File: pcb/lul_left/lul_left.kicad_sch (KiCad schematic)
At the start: 42 parts, among them J1 JST Connector, J2 JST Connector, SW1 SW_Push, SW10 SW_Push, SW11 SW_Push, SW12 SW_Push, SW13 SW_Push, SW14 SW_Push, SW15 SW_Push, SW16 SW_Push, SW17 SW_Push, SW18 SW_Push, SW19 SW_Push, SW2 SW_Push, SW20 SW_Push, SW21 SW_Push, SW22 SW_Push, SW23 SW_Push, SW24 SW_Push, SW25 SW_Push, SW26 SW_Push, SW27 SW_Push, SW28 SW_Push, SW29 SW_Push, SW3 SW_Push, SW30 SW_Push, SW31 SW_Push, SW32 SW_Push, SW33 SW_Push, SW34 SW_Push, SW4 SW_Push, SW5 SW_Push, SW6 SW_Push, SW7 SW_Push, SW8 SW_Push, SW9 SW_Push, U1 nice_nano, U2 nice_nano

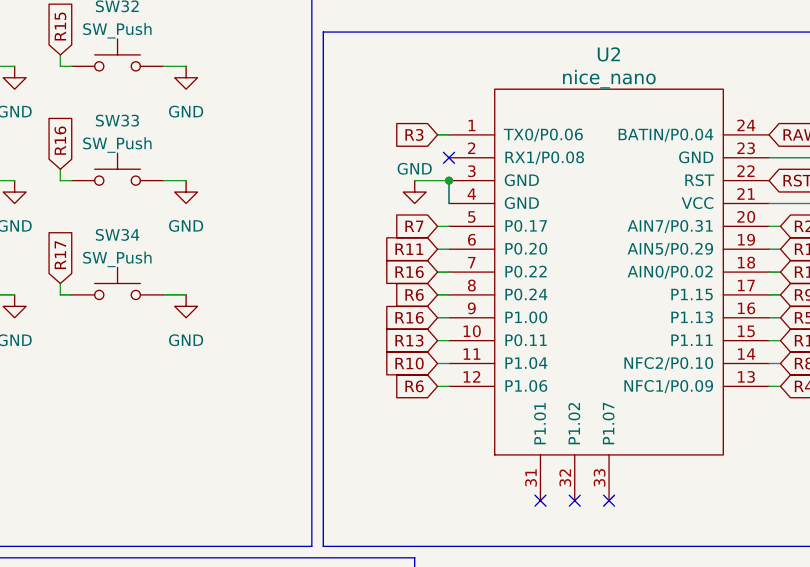
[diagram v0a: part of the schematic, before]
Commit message: fix small connection issue
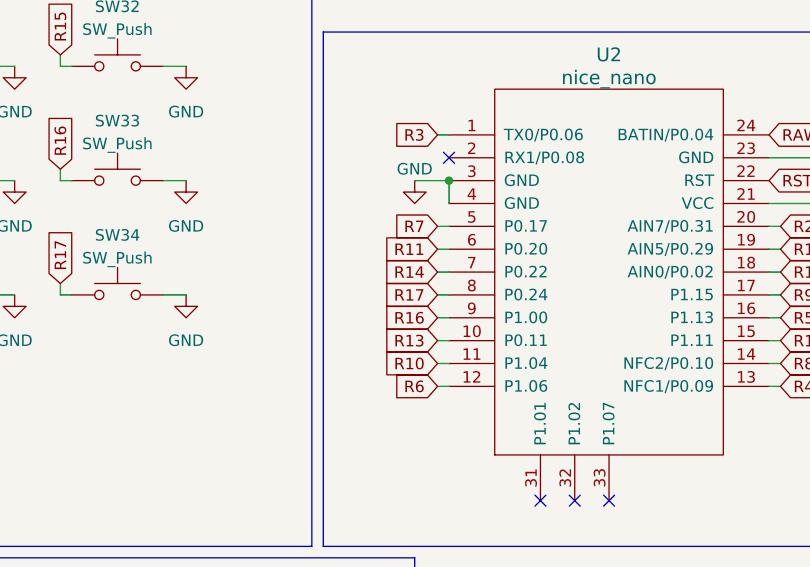
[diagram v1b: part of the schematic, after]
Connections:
- net R14: now also U2.7 (P0.22)
- net R16: no longer U2.7 (P0.22)
- net R17: now also U2.8 (P0.24)
- net R6: no longer U2.8 (P0.24)
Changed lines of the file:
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@@
     )
   )
-  (global_label "R16" (shape input) (at 142.24 111.76 180) (fields_autoplaced)
+  (global_label "R14" (shape input) (at 142.24 111.76 180) (fields_autoplaced)
     (effects (font (size 1.27 1.27)) (justify right))
     (property "Intersheetrefs" "${INTERSHEET_REFS}" (at 135.6452 111.76 0)
@@
     )
   )
-  (global_label "R6" (shape input) (at 142.24 114.3 180) (fields_autoplaced)
+  (global_label "R17" (shape input) (at 142.24 114.3 180) (fields_autoplaced)
     (effects (font (size 1.27 1.27)) (justify right))
-    (property "Intersheetrefs" "${INTERSHEET_REFS}" (at 136.8547 114.3 0)
+    (property "Intersheetrefs" "${INTERSHEET_REFS}" (at 135.6452 114.3 0)
       (effects (font (size 1.27 1.27)) (justify right) hide)
     )
